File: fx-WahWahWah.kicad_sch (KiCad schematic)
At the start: 40 parts, among them J1 Conn_01x10, Q1 2N5088, Q2 2N5089, SW1 ON-ON

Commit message: Some final silk cleanups
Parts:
- C26: footprint Capacitor_THT:C_Rect_L7.2mm_W5.5mm_P5.00mm_FKS2_FKP2_MKS2_MKP2 -> Capacitor_THT:C_Rect_L7.2mm_W4.5mm_P5.00mm_FKS2_FKP2_MKS2_MKP2
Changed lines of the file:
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@@
 			)
 		)
-		(property "Footprint" "Capacitor_THT:C_Rect_L7.2mm_W5.5mm_P5.00mm_FKS2_FKP2_MKS2_MKP2"
+		(property "Footprint" "Capacitor_THT:C_Rect_L7.2mm_W4.5mm_P5.00mm_FKS2_FKP2_MKS2_MKP2"
 			(at 69.85 114.3 0)
 			(hide yes)

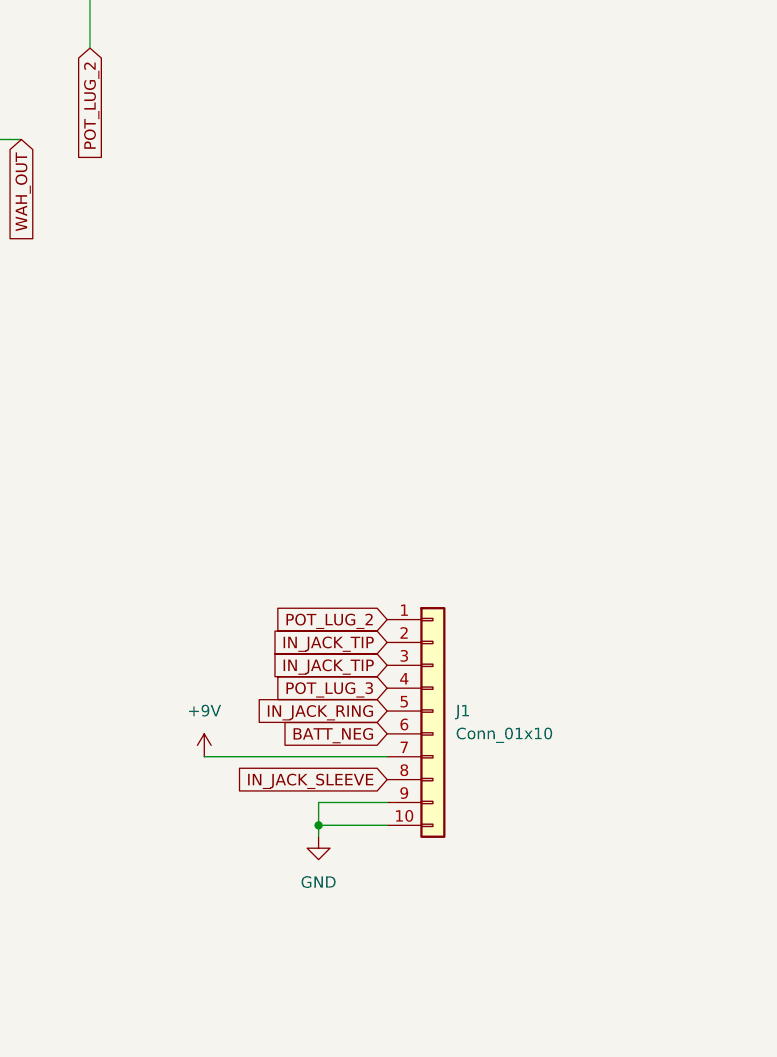
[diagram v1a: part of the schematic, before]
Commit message: fx-WahWahWah v0.3 fab outputs (g3)
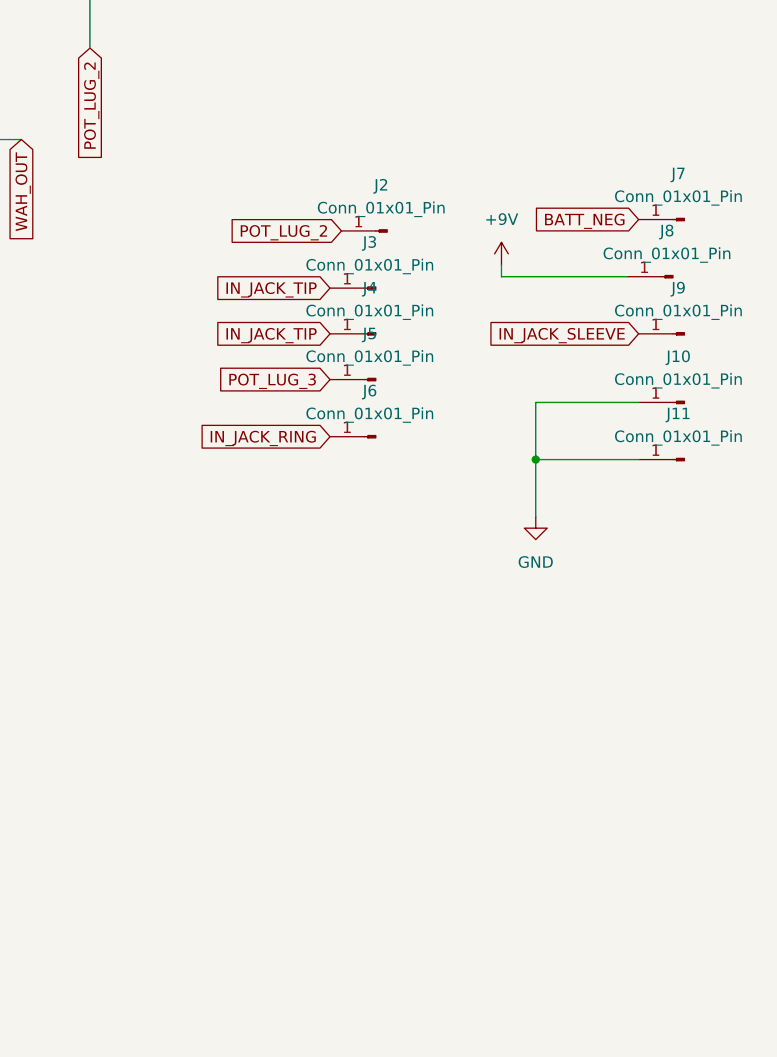
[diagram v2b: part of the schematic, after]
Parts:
- removed J1: Conn_01x10, Connector_PinHeader_2.54mm:PinHeader_1x10_P2.54mm_Vertical, symbol Connector_Generic:Conn_01x10
- added J10, J11, J2, J3, J4, J5, J6, J7, J8, J9: Conn_01x01_Pin, TestPoint:Vector T46-5-9M, symbol Connector:Conn_01x01_Pin
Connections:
- net +9V: now also J8.1 (Pin_1)
- net BATT_NEG: now also J6.1 (Pin_1), J7.1 (Pin_1)
- net GND: now also J10.1 (Pin_1), J11.1 (Pin_1), J9.1 (Pin_1)
- net IN_JACK_TIP: now also J3.1 (Pin_1), J4.1 (Pin_1)
- net POT_LUG_2: now also J2.1 (Pin_1)
- net POT_LUG_3: now also J5.1 (Pin_1)
